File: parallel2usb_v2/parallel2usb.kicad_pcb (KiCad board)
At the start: 4 copper layers, 65.3 x 53.6 mm, 45 parts, among them J1 DB25_Male_MountingHoles, J2 Conn_01x20, U1 74LVC161284DL, U2 Pico

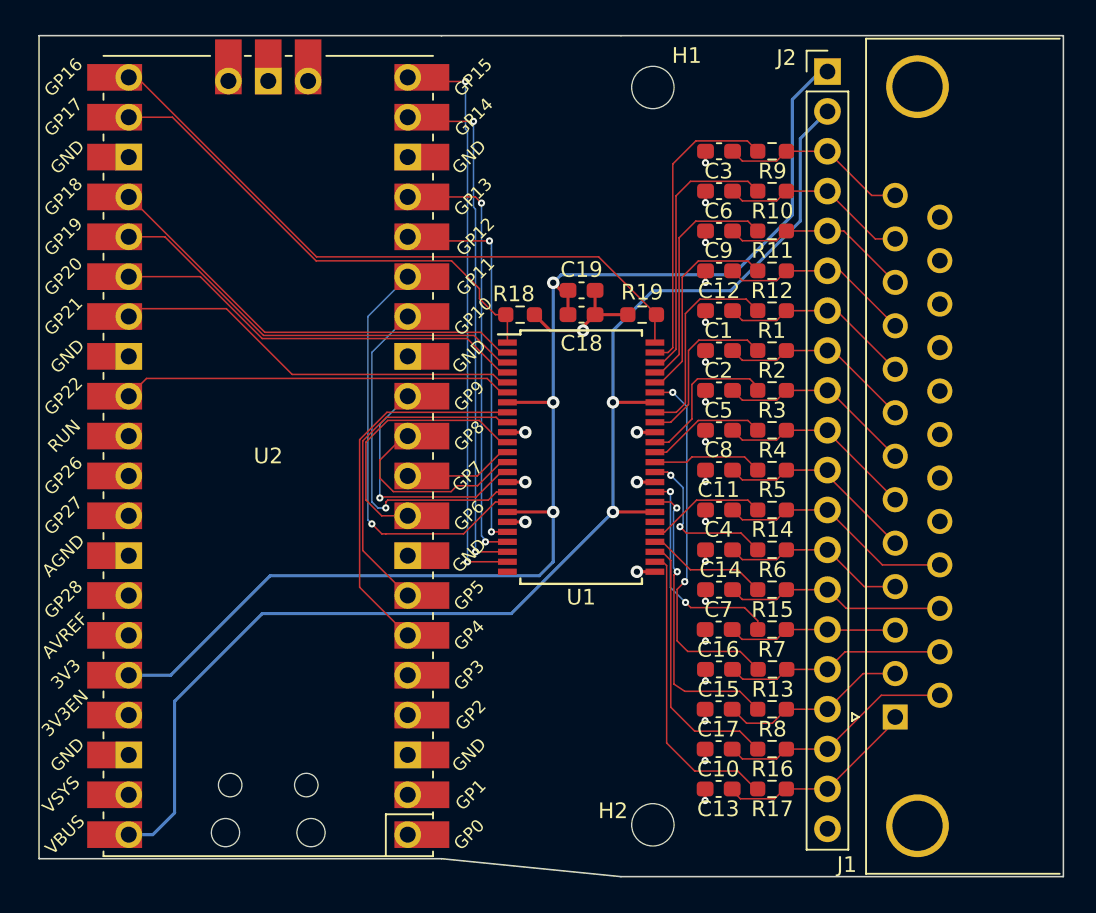
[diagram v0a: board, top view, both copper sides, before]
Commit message: PCB v2.
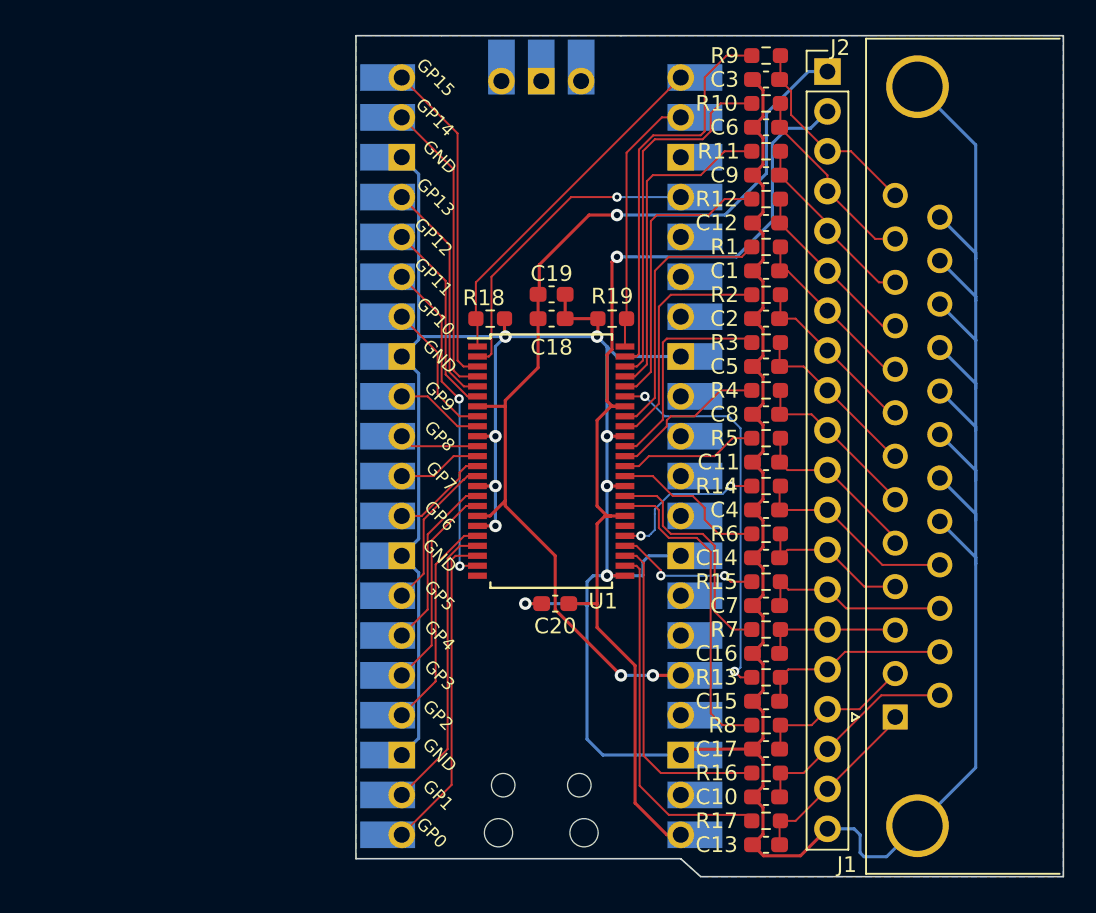
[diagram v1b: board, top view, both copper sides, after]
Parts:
- removed H1, H2: MountingHole, MountingHole:MountingHole_2.7mm_M2.5
- added C20: 100n, Capacitor_SMD:C_0603_1608Metric_Pad1.08x0.95mm_HandSolder, F.Cu at (177.4, 111.0)
- U2: moved to B.Cu
- moved U2 17.4 mm to (176.5, 101.6), turned to 0 degrees
- moved REF** 15.5 mm to (178.7, 101.7)
- moved R9 6.11 mm to (190.9, 76.1)
- moved R10 5.60 mm to (190.9, 79.1)
- moved C3 5.47 mm to (190.9, 77.6)
- moved R11 5.09 mm to (190.9, 82.2)
- moved C6 5.05 mm to (190.9, 80.6)
- moved C13 4.67 mm to (190.9, 126.4)
- moved C9 4.65 mm to (190.9, 83.7)
- moved R12 4.59 mm to (190.9, 85.2)
- moved C10 4.29 mm to (190.9, 123.3)
- moved C12 4.27 mm to (190.9, 86.7)
- moved R1 4.08 mm to (190.9, 88.3)
- moved C17 3.95 mm to (190.9, 120.3)
- moved C1 3.93 mm to (190.9, 89.8)
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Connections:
- U2 pad 1: unconnected-(U2-Pad1) -> /AUTOF_3
- U2 pad 11: /D3_3 -> /D5_3
- U2 pad 12: /D2_3 -> /D6_3
- U2 pad 14: /D1_3 -> /D7_3
- U2 pad 15: /D0_3 -> /STROBE_3
- U2 pad 16: /SELIN_3 -> /ERROR_3
- U2 pad 17: /INIT_3 -> /ACK_3
- U2 pad 19: /AUTOF_3 -> /BUSY_3
- U2 pad 2: unconnected-(U2-Pad2) -> /INIT_3
- U2 pad 20: /STROBE_3 -> /PE_3
- U2 pad 21: /DIR -> /HD
- U2 pad 22: /HD -> /DIR
- U2 pad 25: /PE_3 -> unconnected-(U2-Pad25)
- U2 pad 26: /BUSY_3 -> unconnected-(U2-Pad26)
- U2 pad 27: /ACK_3 -> unconnected-(U2-Pad27)
- U2 pad 29: /ERROR_3 -> unconnected-(U2-Pad29)
- U2 pad 4: unconnected-(U2-Pad4) -> /SELIN_3
- U2 pad 5: unconnected-(U2-Pad5) -> /D0_3
- U2 pad 6: /D7_3 -> /D1_3
- U2 pad 7: /D6_3 -> /D2_3
- U2 pad 9: /D5_3 -> /D3_3
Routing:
- net GND: track 339.0 -> 281.2 mm, vias 24 -> 9
- net /DIR: track 41.7 -> 16.8 mm
- net +3.3V: track 83.7 -> 63.6 mm
- net +5V: track 83.0 -> 66.0 mm, vias 2 -> 1
- net /STROBE_3: track 37.0 -> 21.1 mm
- net /D6_3: track 21.0 -> 5.61 mm
- net /D7_3: track 23.9 -> 9.02 mm
- net /D0_3: track 26.7 -> 13.2 mm, vias 1 -> 0
- net /AUTOF_3: track 33.8 -> 20.6 mm, vias 2 -> 0
- net /ERROR_3: track 25.0 -> 12.5 mm
- net /D5_3: track 16.9 -> 5.09 mm
- net /ACK_3: track 26.3 -> 14.6 mm
- net /SELIN_3: track 24.9 -> 13.9 mm, vias 2 -> 0
- net /D1_3: track 22.2 -> 11.3 mm, vias 1 -> 0
- net /INIT_3: track 28.0 -> 18.5 mm, vias 2 -> 0
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- added copper zone on B.Cu, net GND
- removed copper zone on In2.Cu, net GND
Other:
- board size 65.3 x 53.6 mm -> 45.1 x 53.6 mm
- copper layers 4 -> 2
- board text added: "AF"
- board text added: "BSY"
- board text added: "ERR"
- board text added: "SELI"
- board text added: "STB"
- board text removed: "AUTOF"
- board text removed: "BUSY"
- board text removed: "ERROR"
- board text removed: "SELINT"
- board text removed: "STROBE"
